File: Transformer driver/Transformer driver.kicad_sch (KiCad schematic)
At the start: 8 parts, among them Q2 STGP7NC60HD, U1 PIC18F14K50-ESS, U2 LM393

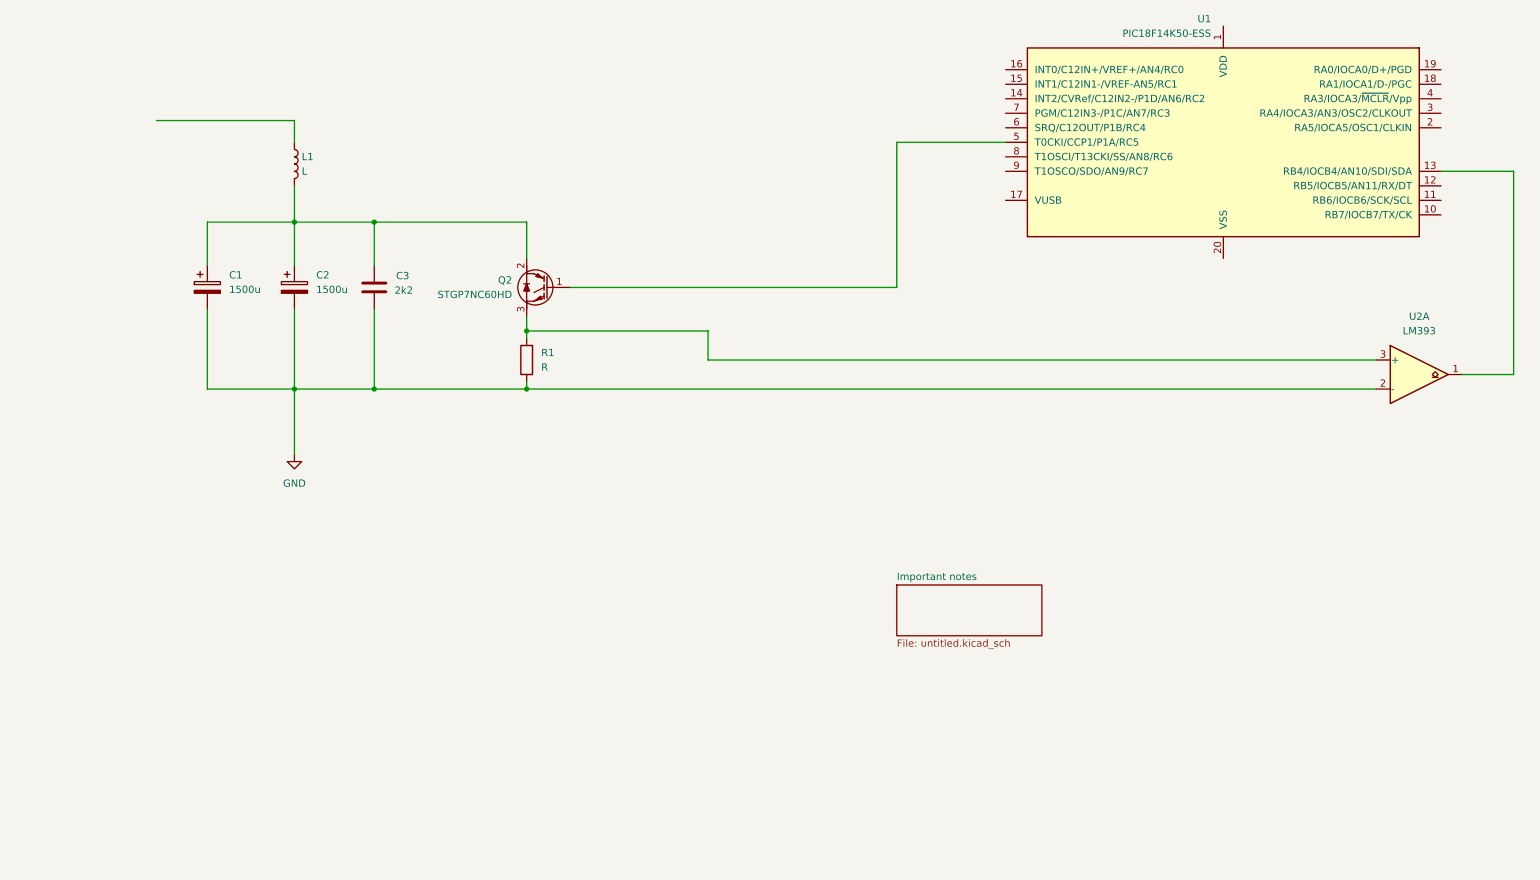
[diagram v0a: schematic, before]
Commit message: second commit
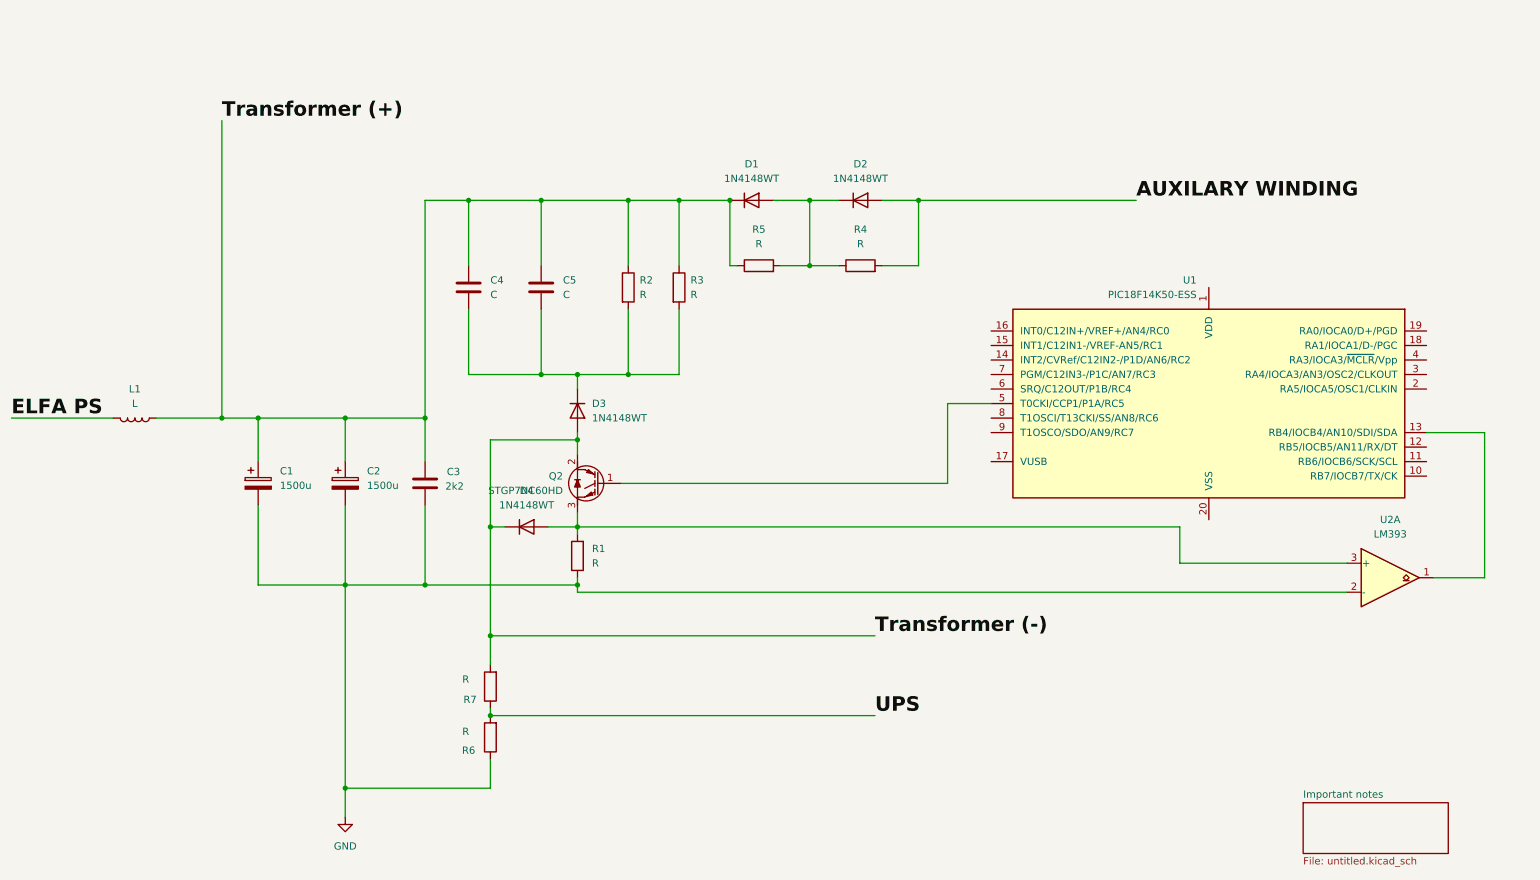
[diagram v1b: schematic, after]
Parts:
- added C4, C5: C, symbol Device:C
- added D1, D2, D3, D4: 1N4148WT, Diode_SMD:D_SOD-523, symbol Diode:1N4148WT
- added R2, R3, R4, R5, R6, R7: R, symbol Device:R
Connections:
- net GND: now also R6.1
- net at Q2.3 (E), R1.2, U2.3 (+): now also D4.2 (A)
- net Transformer (+): now reaches C1.1, C2.1, C3.1
- net Transformer (+): now also L1.1, C4.1, C5.1, D1.1 (K), R2.1, R3.1, R5.1; no longer L1.2, Q2.2 (C)
- new net: D1.2 (A), D2.1 (K), R4.1, R5.2
- new net: C4.2, C5.2, D3.1 (K), R2.2, R3.2
- new net AUXILARY WINDING: D2.2 (A), R4.2
- new net ELFA PS: L1.2
- new net Transformer (-): D3.2 (A), D4.1 (K), Q2.2 (C), R7.2
- new net UPS: R6.2, R7.1
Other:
- moved on the sheet: C1, C2, C3, L1, Q2, R1, U1, U2A

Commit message: commits
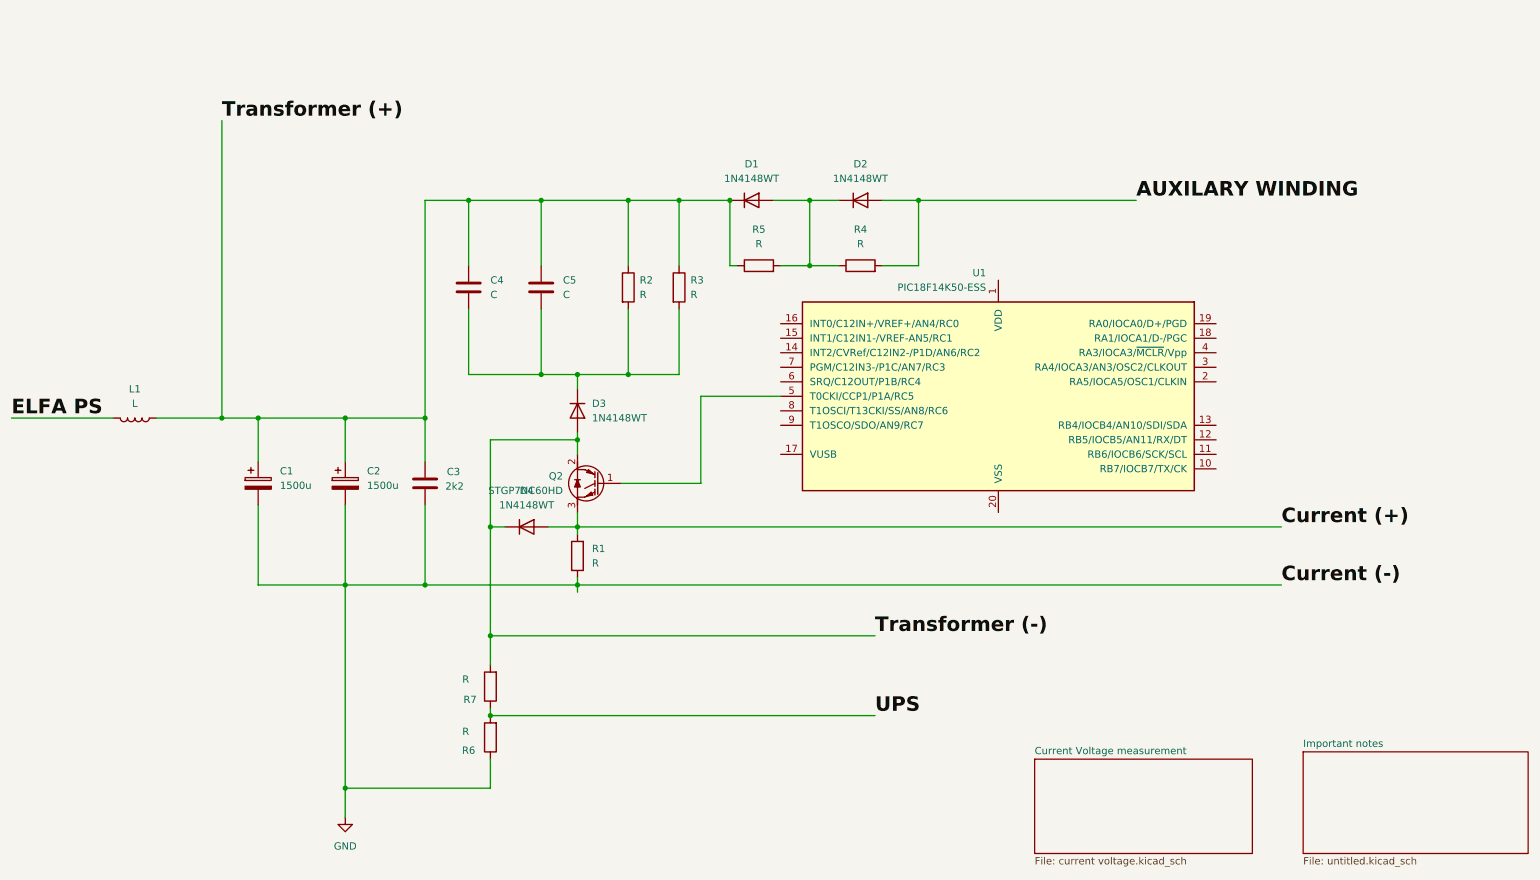
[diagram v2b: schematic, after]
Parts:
- removed U2: LM393, symbol Comparator:LM393
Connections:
- net Current (+): now reaches D4.2 (A), Q2.3 (E), R1.2
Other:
- added sheet Current Voltage measurement (current voltage.kicad_sch)
- moved on the sheet: U1
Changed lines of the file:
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@@
+	(wire
+		(pts
+			(xy 114.3 102.87) (xy 237.49 102.87)
+		)
+		(stroke
+			(width 0)
+			(type default)
+		)
+	)
 	(wire
 		(pts
@@
 	(wire
 		(pts
-			(xy 114.3 102.87) (xy 219.71 102.87)
-		)
-		(stroke
-			(width 0)
-			(type default)
-		)
-	)
-	(wire
-		(pts
 			(xy 154.94 57.15) (xy 149.86 57.15)
 		)
@@
 	(wire
 		(pts
-			(xy 219.71 102.87) (xy 219.71 109.22)
-		)
-		(stroke
-			(width 0)
-			(type default)
-		)
-	)
-	(wire
-		(pts
 			(xy 148.59 45.72) (xy 154.94 45.72)
 		)
@@
 	(wire
 		(pts
-			(xy 273.05 86.36) (xy 273.05 111.76)
-		)
-		(stroke
-			(width 0)
-			(type default)
-		)
-	)
-	(wire
-		(pts
-			(xy 186.69 81.28) (xy 179.07 81.28)
+			(xy 149.86 80.01) (xy 135.89 80.01)
 		)
 		(stroke
@@
 	(wire
 		(pts
-			(xy 121.92 95.25) (xy 179.07 95.25)
+			(xy 121.92 95.25) (xy 135.89 95.25)
 		)
 		(stroke
@@
 	(wire
 		(pts
-			(xy 179.07 81.28) (xy 179.07 95.25)
+			(xy 135.89 80.01) (xy 135.89 95.25)
 		)
 		(stroke
@@
 	(wire
 		(pts
-			(xy 219.71 109.22) (xy 248.92 109.22)
+			(xy 114.3 113.03) (xy 237.49 113.03)
 		)
 		(stroke
@@
 	(wire
 		(pts
-			(xy 273.05 111.76) (xy 264.16 111.76)
-		)
-		(stroke
-			(width 0)
-			(type default)
-		)
-	)
-	(wire
-		(pts
 			(xy 95.25 45.72) (xy 107.95 45.72)
 		)
@@
 	(wire
 		(pts
-			(xy 262.89 86.36) (xy 273.05 86.36)
-		)
-		(stroke
-			(width 0)
-			(type default)
-		)
-	)
-	(wire
-		(pts
 			(xy 58.42 83.82) (xy 58.42 91.44)
 		)
@@
 		(pts
 			(xy 123.19 45.72) (xy 107.95 45.72)
-		)
-		(stroke
-			(width 0)
-			(type default)
-		)
-	)
-	(wire
-		(pts
-			(xy 114.3 114.3) (xy 248.92 114.3)
 		)
 		(stroke
@@
 		)
 	)
+	(label "Current (-)"
+		(at 237.49 113.03 0)
+		(effects
+			(font
+				(size 2.54 2.54)
+				(thickness 0.508)
+				(bold yes)
+				(color 255 46 22 1)
+			)
+			(justify left bottom)
+		)
+	)
 	(label "Transformer (-)"
 		(at 166.37 121.92 0)
@@
 		)
 	)
+	(label "Current (+)"
+		(at 237.49 102.87 0)
+		(effects
+			(font
+				(size 2.54 2.54)
+				(thickness 0.508)
+				(bold yes)
+				(color 255 46 22 1)
+			)
+			(justify left bottom)
+		)
+	)
 	(label "UPS"
 		(at 166.37 135.89 0)
@@
 			)
 			(justify left bottom)
-		)
-	)
-	(symbol
-		(lib_id "Comparator:LM393")
-		(at 256.54 111.76 0)
-		(unit 1)
-		(exclude_from_sim no)
-		(in_bom yes)
-		(on_board yes)
-		(dnp no)
-		(fields_autoplaced yes)
-		(property "Reference" "U2"
-			(at 256.54 101.6 0)
-			(effects
-				(font
-					(size 1.27 1.27)
-				)
-			)
-		)
-		(property "Value" "LM393"
-			(at 256.54 104.14 0)
-			(effects
-				(font
-					(size 1.27 1.27)
-				)
-			)
-		)
-		(property "Footprint" ""
-			(at 256.54 111.76 0)
-			(effects
-				(font
-					(size 1.27 1.27)
-				)
-				(hide yes)
-			)
-		)
-		(property "Datasheet" "http://www.ti.com/lit/ds/symlink/lm393.pdf"
-			(at 256.54 111.76 0)
-			(effects
-				(font
-					(size 1.27 1.27)
-				)
-				(hide yes)
-			)
-		)
-		(property "Description" "Low-Power, Low-Offset Voltage, Dual Comparators, DIP-8/SOIC-8/TO-99-8"
-			(at 256.54 111.76 0)
-			(effects
-				(font
-					(size 1.27 1.27)
-				)
-				(hide yes)
-			)
-		)
-		(pin "2"
-		)
-		(pin "3"
-		)
-		(pin "6"
-		)
-		(pin "1"
-		)
-		(pin "5"
-		)
-		(pin "7"
-		)
-		(pin "8"
-		)
-		(pin "4"
-		)
-		(instances
-			(project ""
-				(path "/efea7640-0212-4c6b-8921-76f5a7157804"
-					(reference "U2")
-					(unit 1)
-				)
-			)
 		)
 	)
@@
 	(symbol
 		(lib_id "MCU_Microchip_PIC18:PIC18F14K50-ESS")
-		(at 224.79 81.28 0)
+		(at 187.96 80.01 0)
 		(mirror y)
 		(unit 1)
@@
 		(dnp no)
 		(property "Reference" "U1"
-			(at 222.6467 59.69 0)
+			(at 185.8167 58.42 0)
 			(effects
 				(font
@@
 		)
 		(property "Value" "PIC18F14K50-ESS"
-			(at 222.6467 62.23 0)
+			(at 185.8167 60.96 0)
 			(effects
 				(font
@@
 		)
 		(property "Footprint" "Package_SO:SSOP-20_5.3x7.2mm_P0.65mm"
-			(at 224.79 81.28 0)
+			(at 187.96 80.01 0)
 			(effects
 				(font
@@
 		)
 		(property "Datasheet" "http://ww1.microchip.com/downloads/en/devicedoc/41350c.pdf"
-			(at 224.79 78.74 0)
+			(at 187.96 77.47 0)
 			(effects
 				(font
@@
 		)
 		(property "Description" "16K Flash, 768 SRAM, 256 EEPROM, USB, nanoWatt XLP, SSOP20"
-			(at 224.79 81.28 0)
+			(at 187.96 80.01 0)
 			(effects
 				(font
@@
 	)
 	(sheet
-		(at 241.3 151.13)
-		(size 25.4 8.89)
+		(at 194.31 143.51)
+		(size 38.1 16.51)
 		(exclude_from_sim no)
 		(in_bom yes)
@@
 			(color 0 0 0 0.0000)
 		)
+		(property "Sheetname" "Current Voltage measurement"
+			(at 194.31 142.7984 0)
+			(effects
+				(font
+					(size 1.27 1.27)
+				)
+				(justify left bottom)
+			)
+		)
+		(property "Sheetfile" "current voltage.kicad_sch"
+			(at 194.31 160.6046 0)
+			(effects
+				(font
+					(size 1.27 1.27)
+				)
+				(justify left top)
+			)
+		)
+		(instances
+			(project "Transformer driver"
+				(path "/efea7640-0212-4c6b-8921-76f5a7157804"
+					(page "3")
+				)
+			)
+		)
+	)
+	(sheet
+		(at 241.3 142.24)
+		(size 39.37 17.78)
+		(exclude_from_sim no)
+		(in_bom yes)
+		(on_board yes)
+		(dnp no)
+		(fields_autoplaced yes)
+		(stroke
+			(width 0.1524)
+			(type solid)
+		)
+		(fill
+			(color 0 0 0 0.0000)
+		)
 		(property "Sheetname" "Important notes"
-			(at 241.3 150.4184 0)
-			(effects
-				(font
+			(at 241.3 141.5284 0)
+			(effects
+				(font
